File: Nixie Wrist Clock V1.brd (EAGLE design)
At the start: 160 x 100 mm, 35 parts, among them Q1 310mA/60V/1.6Ω, Q2 310mA/60V/1.6Ω, Q3 310mA/60V/1.6Ω, Q4 310mA/60V/1.6Ω, Q5 310mA/60V/1.6Ω, U2 NRF52832, X3 32MHz, X4 32.768kHz

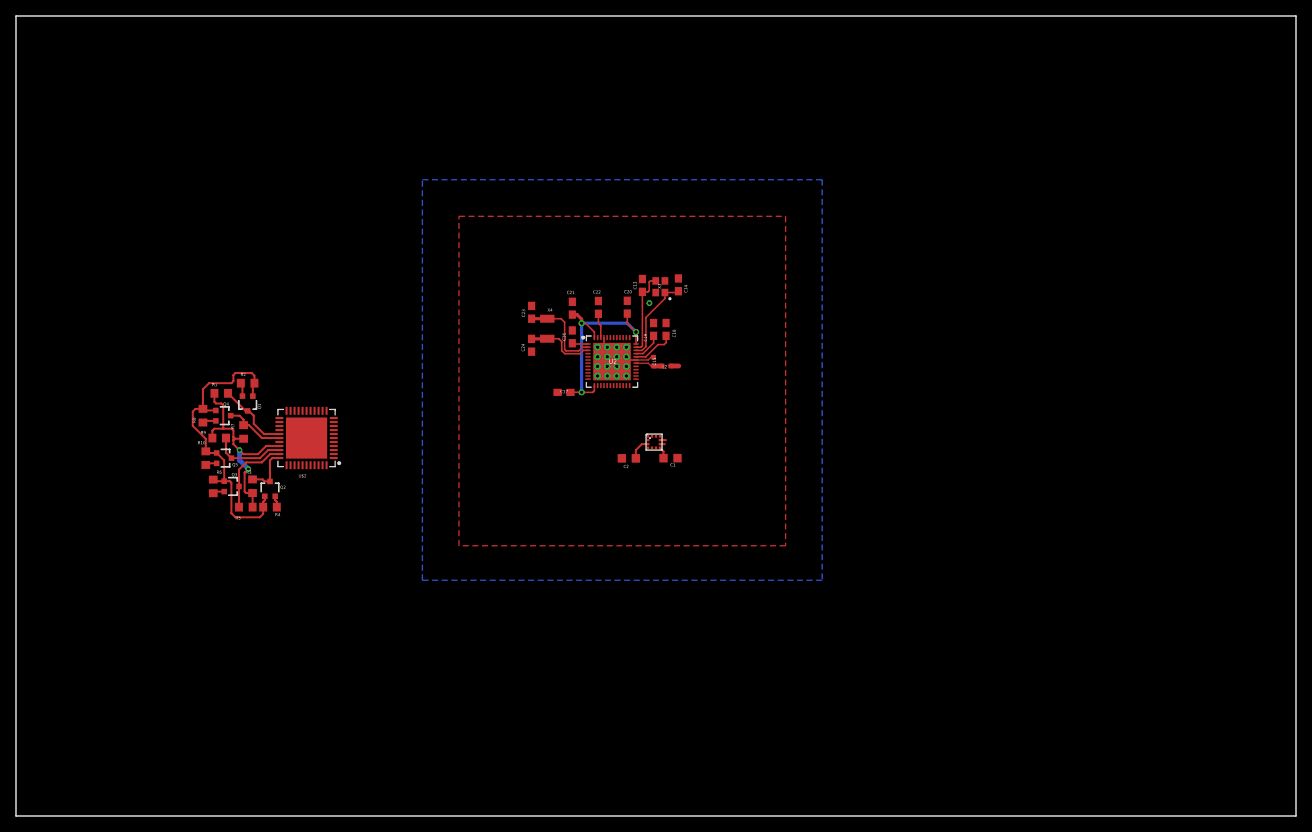
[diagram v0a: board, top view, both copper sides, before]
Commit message: Update (Alp)
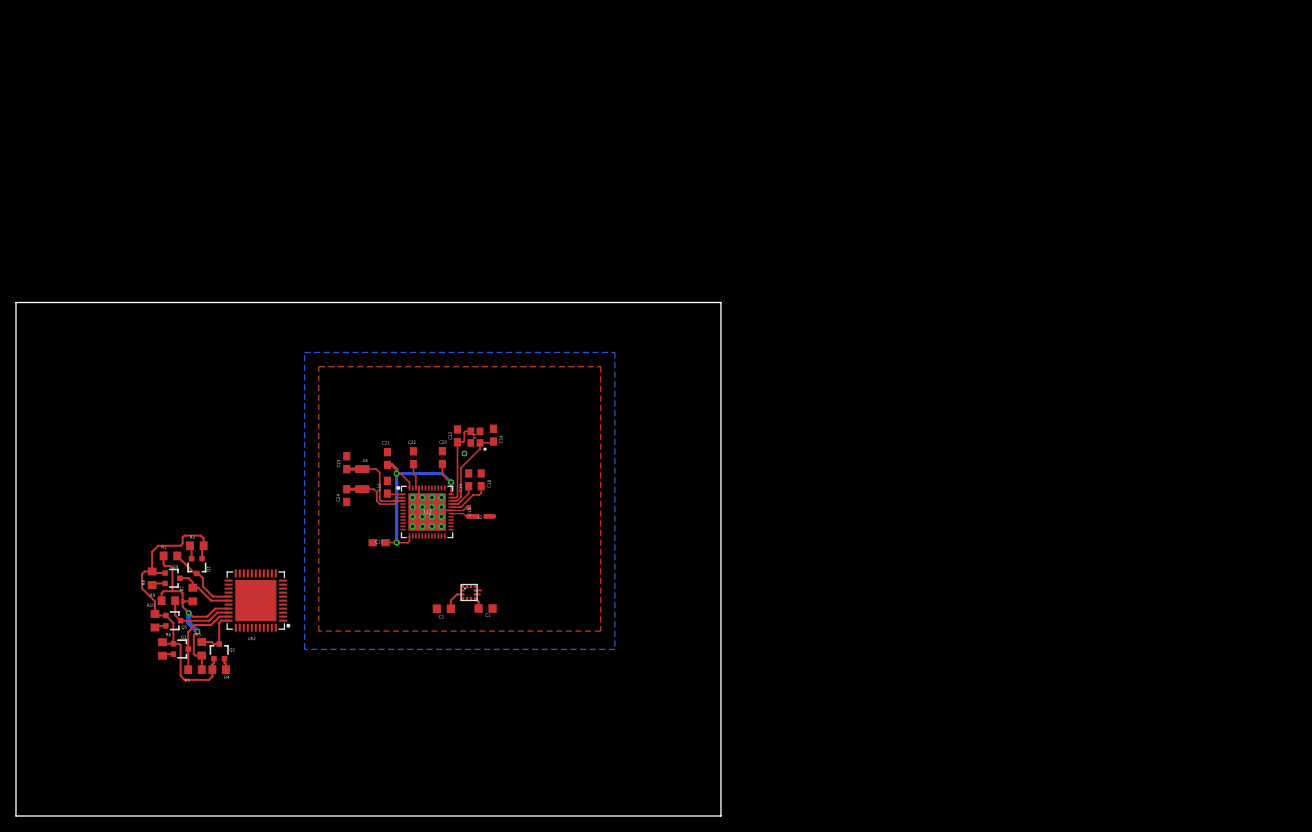
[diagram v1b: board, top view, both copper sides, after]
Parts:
- moved X3 29.8 mm to (57.4, 47.4)
- moved C1 29.8 mm to (58.7, 25.9)
- moved C14 29.8 mm to (59.7, 47.6)
- moved C15 29.8 mm to (56.6, 38.0)
- moved C16 29.8 mm to (46.4, 41.1)
- moved C18 29.8 mm to (58.1, 42.0)
- moved C20 29.8 mm to (53.3, 44.8)
- moved X4 29.8 mm to (43.3, 42.1)
- moved C13 29.8 mm to (55.2, 47.5)
- moved C17 29.8 mm to (45.4, 34.2)
- moved C19 29.8 mm to (56.6, 42.0)
- moved C21 29.8 mm to (46.4, 44.7)
- moved C23 29.8 mm to (41.3, 44.2)
- moved L2 29.8 mm to (58.2, 37.5)
- moved U2 29.8 mm to (51.4, 38.0)
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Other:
- board size 160 x 100 mm -> 88.1 x 64.2 mm
